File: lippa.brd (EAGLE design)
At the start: 50 x 80 mm, 109 parts, among them K1 629105136821, X1 B4B-PH-K-S, X2 B4B-PH-K-S, X3 B4B-PH-K-S, X4 B4B-PH-K-S, X5 LIITTIMET_X3815-10, X8 PS-JOYSTICK, Y1 EKE_PTH3.2-6.5SQ, Y2 EKE_PTH3.2-6.5SQ, Y3 EKE_PTH3.2-6.5SQ, Y4 EKE_PTH3.2-6.5SQ

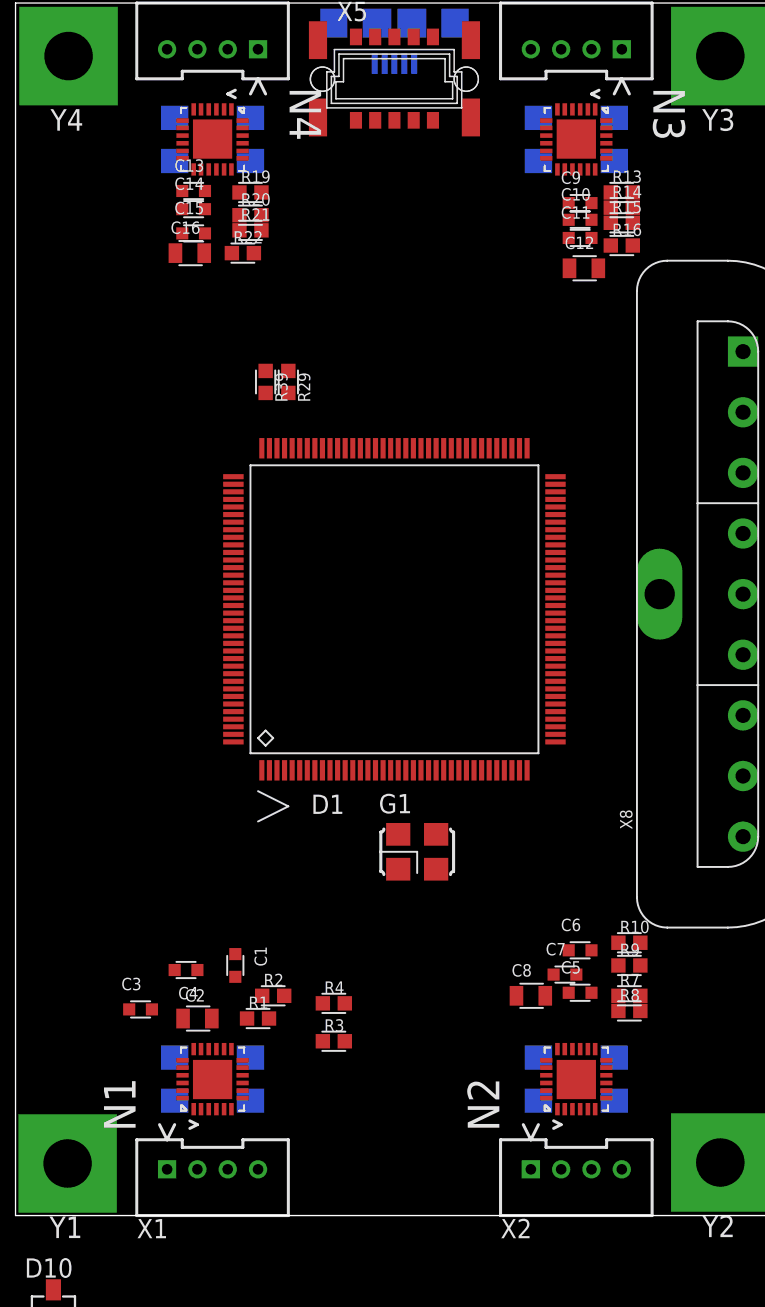
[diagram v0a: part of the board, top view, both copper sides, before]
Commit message: wip
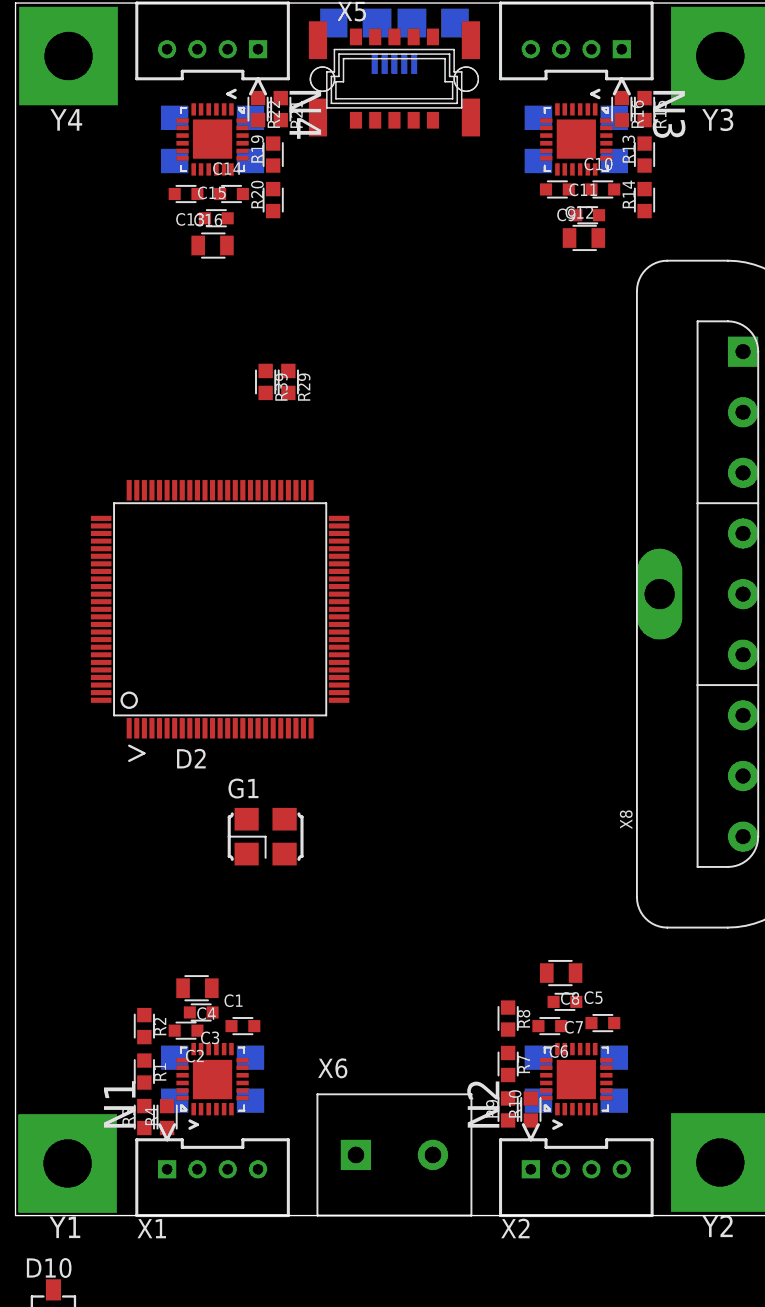
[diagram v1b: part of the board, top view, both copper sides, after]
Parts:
- removed D1: STM32F407ZG, omat_ic_2:LQFP-144
- added D2: STM32F407VE, lippa:LQFP-100
- added X6: (no value), lippa:TE_RUUVILIITIN2
- moved R3 13.5 mm to (8.50, 6.50), turned to 90 degrees
- moved R4 13.3 mm to (10.0, 6.50), turned to 90 degrees
- moved R10 12.8 mm to (34.0, 7.00), turned to 90 degrees
- moved R9 12.4 mm to (32.5, 7.00), turned to 90 degrees
- moved G1 10.0 mm to (16.5, 25.0)
- moved R22 9.55 mm to (16.0, 73.0), turned to 270 degrees
- moved R7 9.18 mm to (32.5, 10.0), turned to 270 degrees
- moved R16 9.00 mm to (40.0, 73.0), turned to 270 degrees
- moved R2 8.73 mm to (8.50, 12.5), turned to 270 degrees
- moved R1 8.28 mm to (8.50, 9.50), turned to 270 degrees
- moved R21 8.25 mm to (17.5, 73.0), turned to 270 degrees
- moved R8 8.02 mm to (32.5, 13.0), turned to 270 degrees
- moved R15 7.65 mm to (41.5, 73.0), turned to 270 degrees
- moved C6 5.39 mm to (35.2, 12.5), turned to 180 degrees
- moved C1 4.03 mm to (15.0, 12.5), turned to 0 degrees
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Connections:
- removed net DIR_4: D1.65
- removed net DIR_5: D1.66
- removed net ENABLE_N: D1.67
- removed net ENA_4: D1.89
- removed net ENA_5: D1.90
- removed net INPUT_0: D1.98
- removed net INPUT_1: D1.99
- removed net INPUT_10: D1.116
- removed net INPUT_11: D1.117
- removed net INPUT_12: D1.118
- removed net INPUT_13: D1.119
- removed net INPUT_14: D1.122
- removed net INPUT_15: D1.123
- removed net INPUT_2: D1.111
- removed net INPUT_3: D1.112
- removed net INPUT_4: D1.113
- removed net INPUT_5: D1.7
- removed net INPUT_8: D1.114
- removed net INPUT_9: D1.115
- removed net N$14: N1.7
- removed net N$15: N1.8
- removed net N$16: N1.9
- removed net N$28: N2.7
- removed net N$29: N2.8
- removed net N$30: N2.9
- removed net N$43: N3.7
- removed net N$44: N3.8
- removed net N$45: N3.9
- removed net N$58: N4.7
- removed net N$59: N4.8
- removed net N$60: N4.9
- removed net OUT_1: D1.26
- removed net OUT_2: D1.27
- removed net OUT_3: D1.69
- removed net OUT_4: D1.70
- removed net PULSE_4: D1.139
- removed net PULSE_5: D1.140
- removed net SERVO_PWM_3: D1.46
- removed net SPARE_1: D1.91
- removed net SPARE_2: D1.92
- new net PULSE_1: D2.63, N2.8
- net +3V3: now also D2.100, D2.11, D2.19, D2.28, D2.50, D2.6, D2.75; no longer D1.108, D1.121, D1.131, D1.143, D1.144, D1.17, D1.30, D1.39, D1.52, D1.6, D1.62, D1.72, D1.84, D1.95
- net +VBAT: now also X6.1
- net BOOT0: now also D2.94; no longer D1.138
- net DIR_0: now also D2.39, N1.9; no longer D1.59
- net DIR_1: now also D2.41, N2.9; no longer D1.60
- net DIR_2: now also D2.42, N3.9; no longer D1.63
- net DIR_3: now also D2.43, N4.9; no longer D1.64
- net ENABLE_PWM_N: now also D2.85; no longer D1.124
- net ENA_0: now also D2.81, N1.7; no longer D1.56
- net ENA_1: now also D2.82, N2.7; no longer D1.57
- net ENA_2: now also D2.83, N3.7; no longer D1.87
- net ENA_3: now also D2.84, N4.7; no longer D1.88
- net GND: now also D2.10, D2.20, D2.27, D2.74, D2.99, X6.2; no longer D1.107, D1.120, D1.130, D1.16, D1.31, D1.38, D1.51, D1.61, D1.83, D1.94
- net I2C1SCL: now also D2.92; no longer D1.136
- net I2C1SDA: now also D2.93; no longer D1.137
- net LED_DEBUG: now also D2.17; no longer D1.28
- net LED_ERR: now also D2.33; no longer D1.44
- net LED_RUN: now also D2.18; no longer D1.29
- net MEAS12V: now also D2.23; no longer D1.34
- net N$62: now also D2.37; no longer D1.48
- net N$63: now also D2.76; no longer D1.109
- net N$73: now also D2.72; no longer D1.105
- net OSCIN: now also D2.12; no longer D1.23
- net OSCOUT: now also D2.13; no longer D1.24
- net PULSE_0: now also D2.59, N1.8; no longer D1.81
- net PULSE_2: now also D2.4, N3.8; no longer D1.96
- net PULSE_3: now also D2.95, N4.8; no longer D1.4
- net RESETL: now also D2.14; no longer D1.25
- net SERVO_PWM_1: now also D2.31; no longer D1.42
- net SERVO_PWM_2: now also D2.32; no longer D1.43
- net SPI1CLK: now also D2.89; no longer D1.133
- net SPI1MISO: now also D2.90; no longer D1.134
- net SPI1MOSI: now also D2.91; no longer D1.135
- net SPI_CS_PS2_N: now also D2.24; no longer D1.35
- net USART1RX: now also D2.69; no longer D1.102
- net USART1TX: now also D2.68; no longer D1.101
- net USART1TXE: now also D2.62; no longer D1.86
- net USART2TX: now also D2.25; no longer D1.36
- net USART3RX: now also D2.56; no longer D1.78
- net USART3TX: now also D2.55; no longer D1.77
- net USBRENUM: now also D2.54; no longer D1.76
- net USB_DM: now also D2.70; no longer D1.103
- net USB_DP: now also D2.71; no longer D1.104
- net VCAP1: now also D2.49; no longer D1.71
- net VCAP2: now also D2.73; no longer D1.106
- net VDDA: now also D2.22; no longer D1.33
- net VREF25: now also D2.21; no longer D1.32

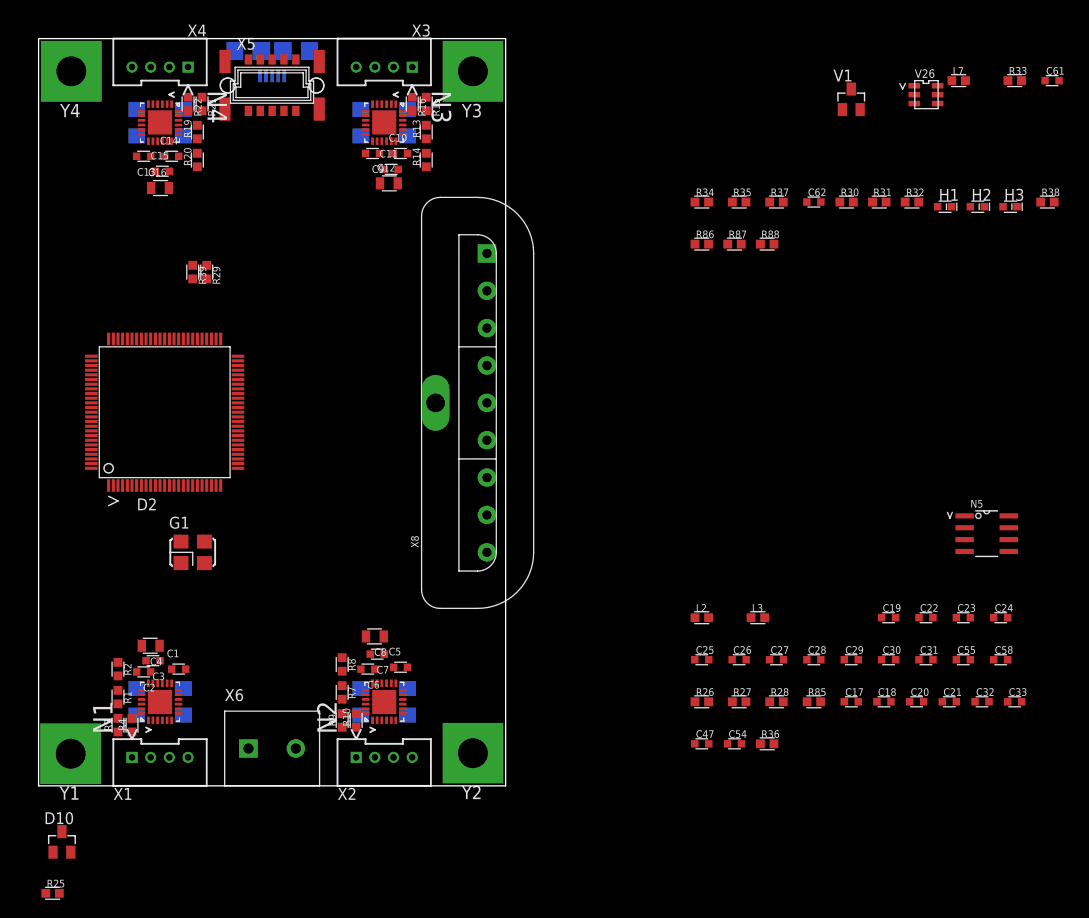
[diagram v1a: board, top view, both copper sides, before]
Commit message: more wip
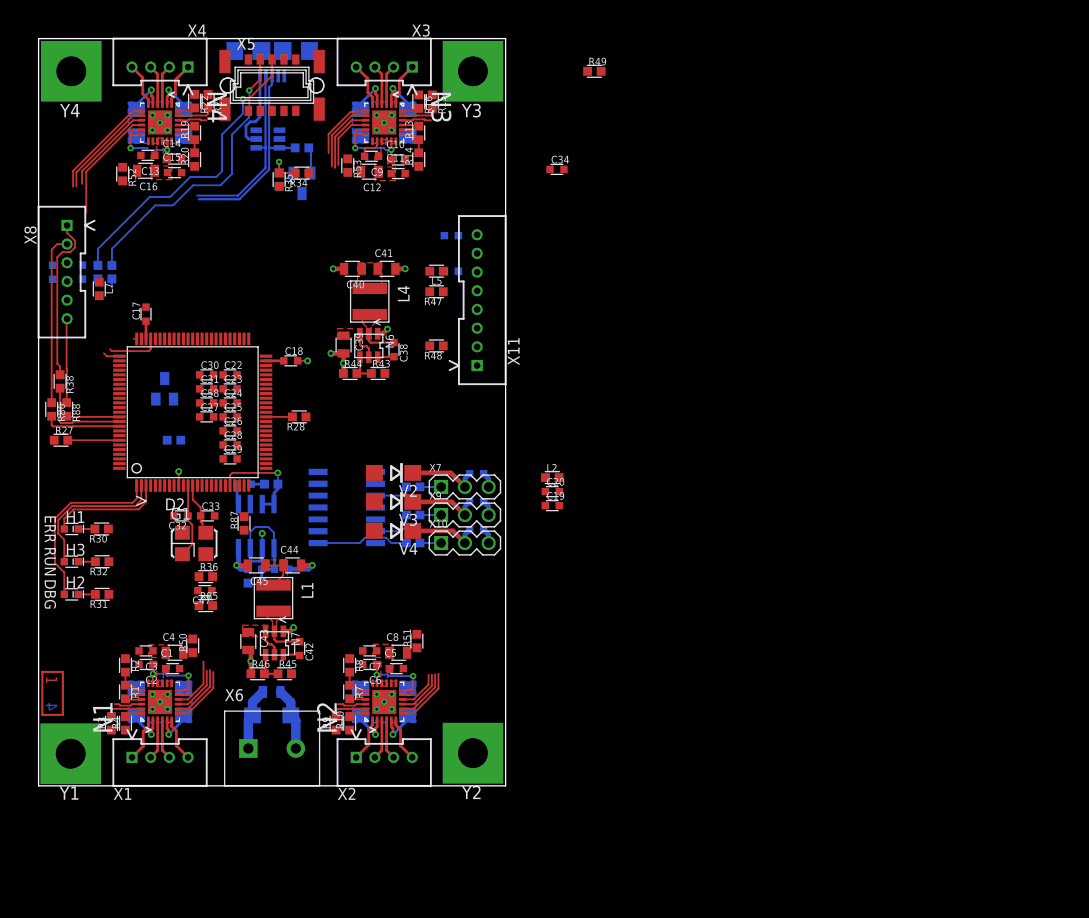
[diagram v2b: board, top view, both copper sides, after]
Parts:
- added C34, C35, C36, C37: (no value), lippa:OMAT_IC_2_C0603
- added C38, C42: 100n 0603, lippa:OMAT_IC_2_C0603
- added C39, C40, C41, C43, C44, C45, C49: 22u 25V, lippa:OMAT_IC_2_C0805
- added C46: 100n, omat_ic_2:C0603
- added C48: 2u2, omat_ic_2:C0603
- added D1: 74AHCT125, lippa:SO14
- added L1: NRS4018-2U2, lippa:NRS4018
- added L4: NRS4018-4U7, lippa:NRS4018
- added L5: IND0603, omat_ic_2:R0603
- added N6, N7: TPS561201, lippa:OMAT_IC_2_SOT23-6
- added R40, R41, R42: (no value), lippa:OMAT_IC_2_R0603
- added R43: 54k9, lippa:OMAT_IC_2_R0603
- added R44, R46: 10k0, lippa:OMAT_IC_2_R0603
- added R45: 33k2, lippa:OMAT_IC_2_R0603
- added R47, R48: (no value), cpu:OMAT_IC_2_R0603
- added R49, R50, R51, R52, R53: 2k00, omat_ic_2:R0603
- added V2, V3, V4: SK34A, lippa:OMAT_IC_2_DO214AC
- added V5: SMAJXXA, lippa:DO214AC
- added X10, X7, X9: PIIKKIRIMA-3, lippa:PIIKKIRIMA-3
- added X11: B8B-PH-K-S, lippa:B8B-PH-K-S
- X8: value PS-JOYSTICK -> B6B-PH-K-S; device cpu:PS-JOYSTICK -> lippa:B6B-PH-K-S
- moved C61 108.9 mm to (1.50, 55.0), flipped to the bottom, turned to 90 degrees
- moved H3 107.4 mm to (3.50, 24.0)
- moved R38 107.4 mm to (2.30, 43.3), turned to 270 degrees
- moved H2 105.5 mm to (3.50, 20.5)
- moved H1 99.7 mm to (3.50, 27.5)
- moved R32 94.9 mm to (6.80, 24.0), turned to 180 degrees
- moved L7 94.7 mm to (6.50, 53.2), turned to 270 degrees
- moved R31 93.2 mm to (6.80, 20.5), turned to 180 degrees
- moved C58 89.3 mm to (18.0, 41.0)
- moved C33 88.7 mm to (18.1, 28.9)
- moved C32 88.0 mm to (15.2, 28.9), turned to 180 degrees
- moved R30 87.1 mm to (6.75, 27.5), turned to 180 degrees
- moved C17 86.2 mm to (11.5, 50.5), turned to 90 degrees
- moved C24 85.6 mm to (20.5, 41.0)
- moved C31 82.3 mm to (18.0, 42.5)
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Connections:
- net MEAS12V renamed MEASVBAT
- net N$62 renamed BOOT1
- net N$63 renamed SWCLK_CPU
- net N$69 renamed DATA
- net N$70 renamed CMD
- net N$73 renamed SWDIO_CPU
- removed net DIR_0: D2.39, N1.9
- removed net ENA_0: D2.81, N1.7
- removed net ENA_1: D2.82, N2.7
- removed net ENA_2: D2.83, N3.7
- removed net ENA_3: D2.84, N4.7
- removed net N$17: C6.1, N2.17
- removed net N$2: C2.1, N1.17
- removed net N$32: C10.1, N3.17
- removed net N$47: C14.1, N4.17
- removed net PULSE_0: D2.59, N1.8
- removed net USART2TX: D2.25
- new net +5V: C34.1, C40.1, C41.1, D1.14, L4.1, L5.2, R43.2
- new net ATT: R87.1, X8.5
- new net CLK: R88.1, X8.6
- new net DIR_4: D2.43, N4.9
- new net ENA_1_N: D2.81, N1.7, R50.1
- new net ENA_2_N: D2.82, N2.7, R51.1
- new net ENA_3_N: D2.83, N3.7, R52.1
- new net ENA_4_N: D2.84, N4.7, R53.1
- new net LIDAR_VCC: C46.1, C48.1, L5.1, X11.6, X11.8
- new net MODE_1: D2.78, N1.10
- new net MODE_2: D2.79, N2.10
- new net MODE_3: D2.80, N3.10
- new net MODE_4: D2.7, N4.10
- new net N$14: R41.2, X9.1
- new net N$15: R40.2, X7.1
- new net N$16: R42.2, X10.1
- new net N$28: D1.3, R40.1
- new net N$29: D1.6, R41.1
- new net N$30: D1.8, R42.1
- new net N$43: C38.1, L4.2, N6.2
- new net N$44: C37.1, V4.C, X10.2
- new net N$45: C36.1, V3.C, X9.2
- new net N$58: C35.1, V2.C, X7.2
- new net N$59: C38.2, N6.6
- new net N$60: N6.4, R43.1, R44.2
- new net N$69: X11.4, X11.7
- new net N$74: C42.1, L1.2, N7.2
- new net N$75: C42.2, N7.6
- new net N$76: N7.4, R45.1, R46.2
- new net PULSE_4: D2.95, N4.8
- new net SERVO_PWM_3: D1.9, D2.35
- new net VINT_1: C2.1, N1.11, N1.12, N1.17
- new net VINT_2: C6.1, N2.11, N2.12, N2.17
- new net VINT_3: C10.1, N3.11, N3.12, N3.17
- new net VINT_4: C14.1, N4.11, N4.12, N4.17
- net +3V3: now also C44.1, C45.1, L1.1, R45.2, R49.2, R50.2, R51.2, R52.2, R53.2
- net +VBAT: now also C39.1, C43.1, C49.1, N6.3, N6.5, N7.3, N7.5, V2.A, V3.A, V4.A, V5.C
- net DIR_1: now also D2.39, N1.9; no longer D2.41, N2.9
- net DIR_2: now also D2.41, N2.9; no longer D2.42, N3.9
- net DIR_3: now also D2.42, N3.9; no longer D2.43, N4.9
- net ENABLE_PWM_N: now also D1.1, D1.10, D1.4, R49.1
- net FAULT_N: now also D2.87
- net GND: now also C34.2, C35.2, C36.2, C37.2, C39.2, C40.2, C41.2, C43.2, C44.2, C45.2, C46.2, C48.2, C49.2, D1.12, D1.13, D1.7, N6.1, N7.1, R44.1, R46.1, V5.A, X10.3, X11.3, X7.3, X8.3, X9.3; no longer X8.4
- net LED_DEBUG: now also D2.1; no longer D2.17
- net LED_ERR: now also D2.3; no longer D2.33
- net LED_RUN: now also D2.2; no longer D2.18
- net N$71: now also R48.1, X11.2; no longer R87.1, X8.6
- net N$72: now also R47.1, X11.5; no longer R88.1, X8.7
- net PSVCC: now also X8.4; no longer X8.5
- net PULSE_1: now also D2.59, N1.8; no longer D2.63, N2.8
- net PULSE_2: now also D2.63, N2.8; no longer D2.4, N3.8
- net PULSE_3: now also D2.4, N3.8; no longer D2.95, N4.8
- net SERVO_PWM_1: now also D1.2
- net SERVO_PWM_2: now also D1.5
- net SLEEP_N: now also D2.86
- net USART1RX: now also R47.2
- net USART1TX: now also R48.2
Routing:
- net GND: track 0.00 -> 43.4 mm, vias 0 -> 32
- net SWCLK: track 0.00 -> 33.0 mm, vias 0 -> 1
- net SWDIO: track 0.00 -> 31.5 mm, vias 0 -> 1
- net USB_DP: track 0.00 -> 21.8 mm
- net LED_DEBUG: track 0.00 -> 19.6 mm
- net USB_DM: track 0.00 -> 19.5 mm
- net CMD: track 0.00 -> 18.3 mm
- net DATA: track 0.00 -> 17.7 mm
- net LED_RUN: track 0.00 -> 16.1 mm
- net N$2: track 0.00 -> 13.6 mm
- net +VBAT: track 0.00 -> 12.9 mm
- net MODE_4: track 0.00 -> 12.4 mm
- net LED_ERR: track 0.00 -> 12.3 mm
- net SLEEP_N: track 0.00 -> 12.2 mm
- net ENA_4_N: track 0.00 -> 11.7 mm
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- added copper zone on layer 1, net +3V3
- added copper zone on layer 1, net +5V
- added copper zone on layer 1, net +VBAT
- added copper zone on layer 15, net GND
- added copper zone on layer 16, net GND
- added copper zone on layer 1, net N$43
- added copper zone on layer 1, net N$74
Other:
- board text added: "1"
- board text added: "2"
- board text added: "3"
- board text added: "4"
- board text added: "DBG"
- board text added: "ERR"
- board text added: "RUN"
